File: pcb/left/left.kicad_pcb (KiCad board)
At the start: 2 copper layers, 31.8 x 72.4 mm, 21 parts, among them J1 Conn_01x07

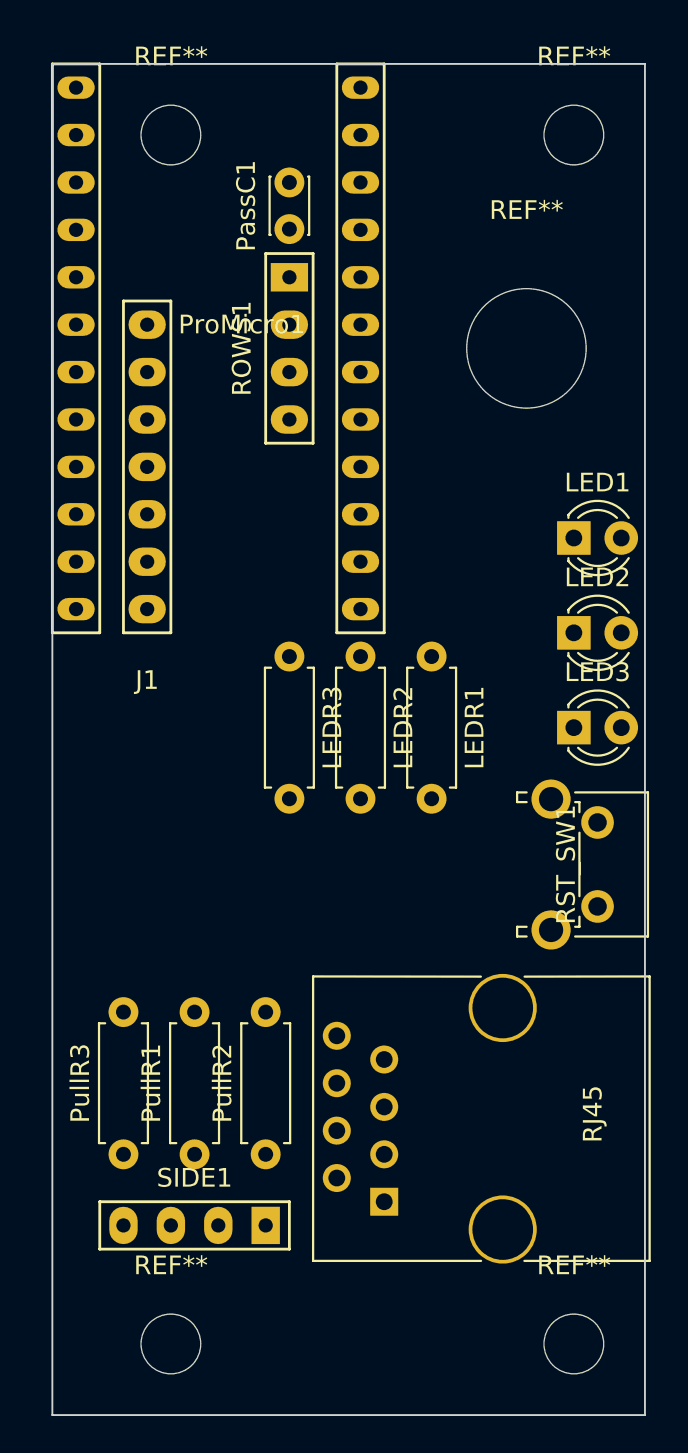
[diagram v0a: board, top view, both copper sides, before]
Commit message: improve pcb size
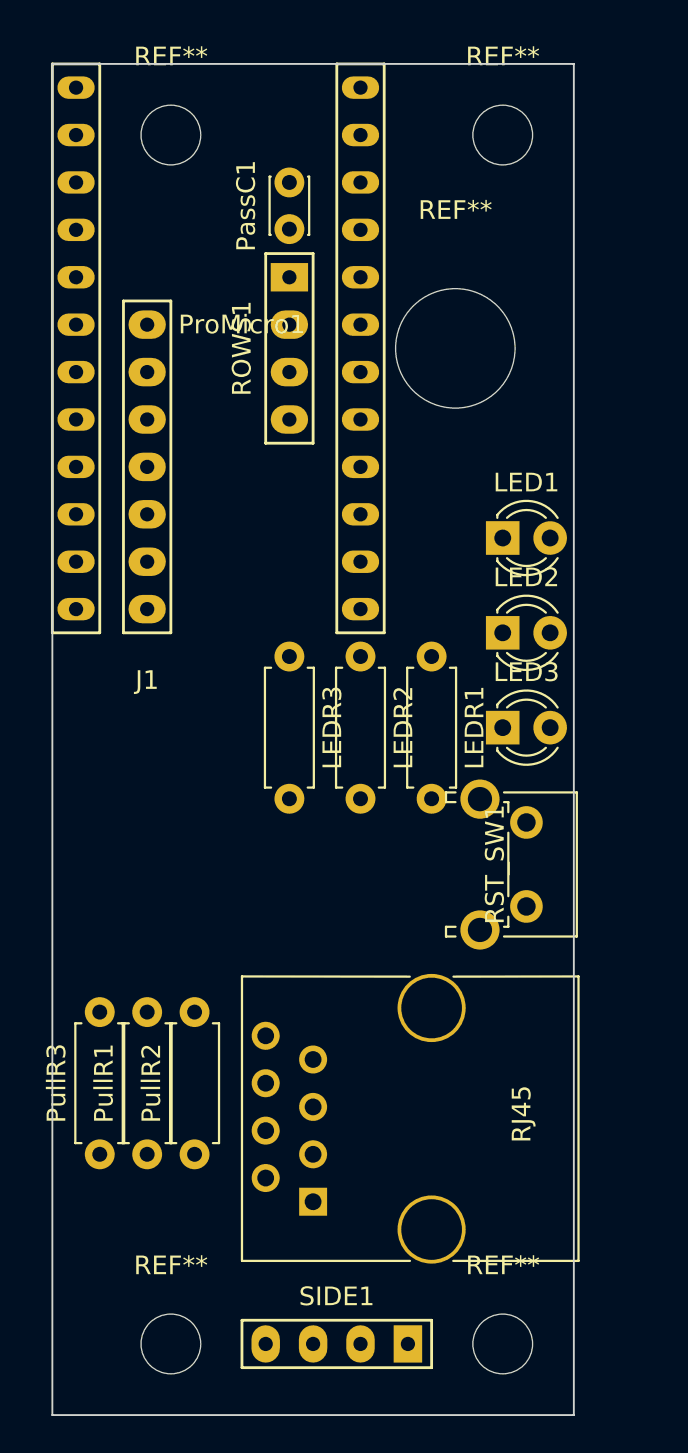
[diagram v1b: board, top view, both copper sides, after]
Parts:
- moved SIDE1 9.92 mm to (47.0, 97.8)
- moved PullR2 3.81 mm to (39.4, 87.6)
- moved RJ45 3.81 mm to (45.7, 90.2)
- moved RST_SW1 3.81 mm to (57.1, 69.8)
- moved LED1 3.81 mm to (55.9, 54.6)
- moved LED2 3.81 mm to (55.9, 59.7)
- moved LED3 3.81 mm to (55.9, 64.8)
- moved REF** 3.81 mm to (55.9, 33.0)
- moved REF** 3.81 mm to (53.3, 44.5)
- moved REF** 3.81 mm to (55.9, 97.8)
- moved PullR1 2.54 mm to (36.8, 87.6)
- moved PullR3 1.27 mm to (34.3, 87.6)
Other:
- board size 31.8 x 72.4 mm -> 27.9 x 72.4 mm
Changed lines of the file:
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@@
     (links 44)
     (no_connects 44)
-    (area 28.539857 27.842 66.710143 103.068)
+    (area 28.539857 27.842 69.250143 103.068)
     (thickness 1.6)
     (drawings 4)
@@
   )
   (module LEDs:LED_D3.0mm (layer F.Cu)
-    (at 59.69 54.61)
+    (at 55.88 54.61)
     (descr "LED, diameter 3.0mm, 2 pins")
     (tags "LED diameter 3.0mm 2 pins")
@@
   )
   (module LEDs:LED_D3.0mm (layer F.Cu)
-    (at 59.69 59.69)
+    (at 55.88 59.69)
     (descr "LED, diameter 3.0mm, 2 pins")
     (tags "LED diameter 3.0mm 2 pins")
@@
   )
   (module LEDs:LED_D3.0mm (layer F.Cu)
-    (at 59.69 64.77)
+    (at 55.88 64.77)
     (descr "LED, diameter 3.0mm, 2 pins")
     (tags "LED diameter 3.0mm 2 pins")
@@
   )
   (module Resistors_THT:R_Axial_DIN0207_L6.3mm_D2.5mm_P7.62mm_Horizontal (layer F.Cu)
-    (at 39.37 87.63 90)
+    (at 36.83 87.63 90)
     (descr "Resistor, Axial_DIN0207 series, Axial, Horizontal, pin pitch=7.62mm, 0.25W = 1/4W, length*diameter=6.3*2.5mm^2, http://cdn-reichelt.de/documents/datenblatt/B400/1_4W%23YAG.pdf")
     (tags "Resistor Axial_DIN0207 series Axial Horizontal pin pitch 7.62mm 0.25W = 1/4W length 6.3mm diameter 2.5mm")
@@
   )
   (module Resistors_THT:R_Axial_DIN0207_L6.3mm_D2.5mm_P7.62mm_Horizontal (layer F.Cu)
-    (at 43.18 87.63 90)
+    (at 39.37 87.63 90)
     (descr "Resistor, Axial_DIN0207 series, Axial, Horizontal, pin pitch=7.62mm, 0.25W = 1/4W, length*diameter=6.3*2.5mm^2, http://cdn-reichelt.de/documents/datenblatt/B400/1_4W%23YAG.pdf")
     (tags "Resistor Axial_DIN0207 series Axial Horizontal pin pitch 7.62mm 0.25W = 1/4W length 6.3mm diameter 2.5mm")
@@
   )
   (module Resistors_THT:R_Axial_DIN0207_L6.3mm_D2.5mm_P7.62mm_Horizontal (layer F.Cu)
-    (at 35.56 87.63 90)
+    (at 34.29 87.63 90)
     (descr "Resistor, Axial_DIN0207 series, Axial, Horizontal, pin pitch=7.62mm, 0.25W = 1/4W, length*diameter=6.3*2.5mm^2, http://cdn-reichelt.de/documents/datenblatt/B400/1_4W%23YAG.pdf")
     (tags "Resistor Axial_DIN0207 series Axial Horizontal pin pitch 7.62mm 0.25W = 1/4W length 6.3mm diameter 2.5mm")
@@
   )
   (module Connectors:RJ45_8 (layer F.Cu)
-    (at 49.53 90.17 90)
+    (at 45.72 90.17 90)
     (tags RJ45)
     (fp_text reference RJ45 (at 4.7 11.18 90) (layer F.SilkS)
@@
   )
   (module Buttons_Switches_THT:SW_Tactile_SPST_Angled_PTS645Vx31-2LFS (layer F.Cu)
-    (at 60.96 69.85 270)
+    (at 57.15 69.85 270)
     (descr "tactile switch SPST right angle, PTS645VL31-2 LFS")
     (tags "tactile switch SPST angled PTS645VL31-2 LFS C&K Button")
@@
   )
   (module 4x6t2:Wirepad_01x04 (layer F.Cu)
-    (at 39.37 91.44 270)
+    (at 46.99 97.79 270)
     (fp_text reference SIDE1 (at -2.54 0 360) (layer F.SilkS)
       (effects (font (size 1 1) (thickness 0.15)))
@@
   )
   (module Mounting_Holes:MountingHole_3.2mm_M3 (layer F.Cu)
-    (at 59.69 33.02)
+    (at 55.88 33.02)
     (descr "Mounting Hole 3.2mm, no annular, M3")
     (tags "mounting hole 3.2mm no annular m3")
@@
   )
   (module Mounting_Holes:MountingHole_6.4mm_M6 (layer F.Cu)
-    (at 57.15 44.45)
+    (at 53.34 44.45)
     (descr "Mounting Hole 6.4mm, no annular, M6")
     (tags "mounting hole 6.4mm no annular m6")
@@
   )
   (module Mounting_Holes:MountingHole_3.2mm_M3 (layer F.Cu)
-    (at 59.69 97.79)
+    (at 55.88 97.79)
     (descr "Mounting Hole 3.2mm, no annular, M3")
     (tags "mounting hole 3.2mm no annular m3")
@@
       (net 6 /COL5))
   )
-  (gr_line (start 31.75 101.6) (end 63.5 101.6) (layer Edge.Cuts) (width 0.1))
-  (gr_line (start 63.5 29.21) (end 63.5 101.6) (layer Edge.Cuts) (width 0.1))
+  (gr_line (start 31.75 101.6) (end 59.69 101.6) (layer Edge.Cuts) (width 0.1))
+  (gr_line (start 59.69 29.21) (end 59.69 101.6) (layer Edge.Cuts) (width 0.1))
   (gr_line (start 31.75 29.21) (end 31.75 101.6) (layer Edge.Cuts) (width 0.1))
-  (gr_line (start 63.5 29.21) (end 31.75 29.21) (layer Edge.Cuts) (width 0.1))
+  (gr_line (start 59.69 29.21) (end 31.75 29.21) (layer Edge.Cuts) (width 0.1))
 )
